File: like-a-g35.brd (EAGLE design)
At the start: 100 x 80 mm, 17 parts, among them J1 AVR_SPI_PRG_62X3_LOCK, Q1 16MHz, X1 S1, X2 S2, X3 S3, X4 POWER

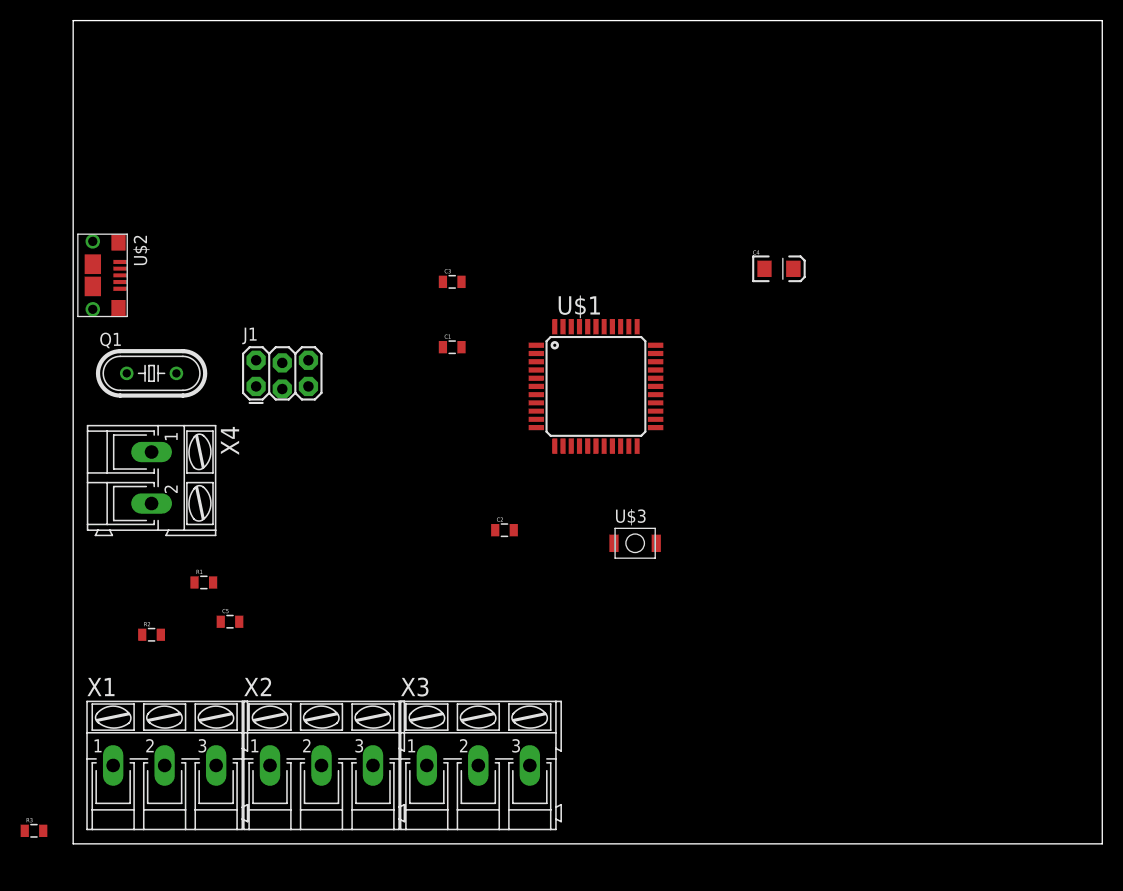
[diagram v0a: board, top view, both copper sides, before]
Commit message: 0.9.
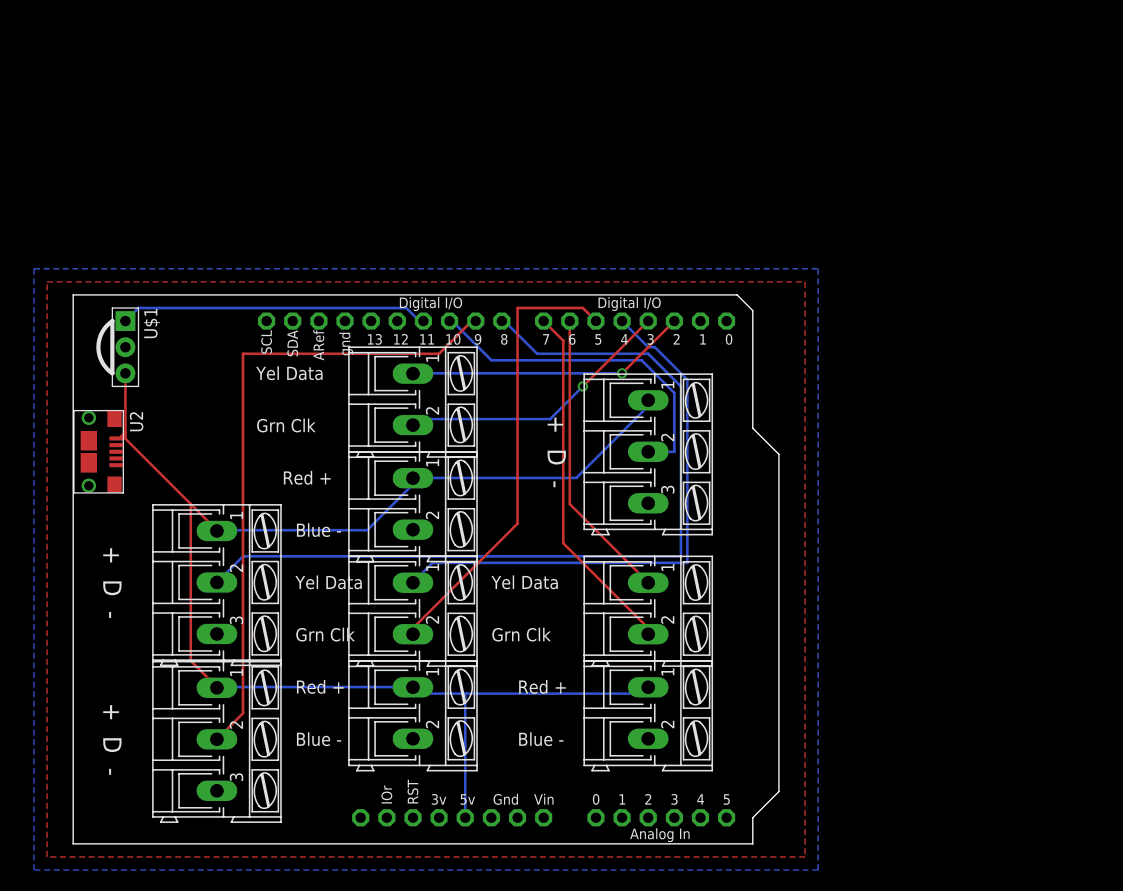
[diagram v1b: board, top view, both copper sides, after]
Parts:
- removed C1, C2: 18pF, programmer:0805
- removed C3, C5: 0.1uF, programmer:0805
- removed C4: 10uF, programmer:EIA3216
- removed J1: AVR_SPI_PRG_62X3_LOCK, programmer:2X3_LOCK
- removed Q1: 16MHz, crystal:HC49/S
- removed R1, R2: 22, like-a-g35:0805
- removed R3: 10K, like-a-g35:0805
- removed U$2: FCI_8193_MICRO_USB, programmer:FCI_MICRO_USB_8193
- removed U$3: BUTTON_TD-85XU, programmer:BUTTON_TD-85XU
- added U1: ARDUINOR3-DIMENSION, adafruit:ARDUINOR3
- added U2: FCI_8193_MICRO_USB, programmer:FCI_MICRO_USB_8193
- added X5, X6: POWER, con-ptr500:AK300/2
- added X7: WS1, con-ptr500:AK300/2
- added X8: WS2, con-ptr500:AK300/2
- added X9: WS3, con-ptr500:AK300/2
- U$1: value ATMEGA32U4-AU -> PNA460XM; device like-a-g35:TQFP44 -> adafruit:PNA460XM
- X1: value S1 -> G1
- X2: value S2 -> G2
- X3: value S3 -> G3
- moved U$1 45.9 mm to (5.08, 48.3), turned to 270 degrees
- moved X3 34.7 mm to (55.9, 38.1), turned to 270 degrees
- moved X4 25.5 mm to (33.0, 33.0)
- moved X1 18.5 mm to (14.0, 25.4), turned to 270 degrees
- moved X2 10.5 mm to (14.0, 10.2), turned to 270 degrees
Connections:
- removed net !RESET: J1.5, U$1.13
- removed net 3V3: C5.1, U$1.6
- removed net D+: R2.2, U$1.4
- removed net D-: R1.2, U$1.3
- removed net MISO: J1.1, U$1.11
- removed net MOSI: J1.4, U$1.10
- removed net N$1: R3.1, U$1.33, U$3.PAD1
- removed net RAW_D+: R2.1, U$2.D+
- removed net RAW_D-: R1.1, U$2.D-
- removed net SCK: J1.3, U$1.9
- removed net XTAL1: C1.1, Q1.2, U$1.17
- removed net XTAL2: C2.1, Q1.1, U$1.16
- new net 3V: U1.3V
- new net CLK1: U1.D3, X7.2
- new net CLK2: U1.D5, X8.2
- new net CLK3: U1.D7, X9.2
- new net DATA1: U1.D2, X7.1
- new net DATA2: U1.D4, X8.1
- new net DATA3: U1.D6, X9.1
- new net GDATA1: U1.D8, X1.2
- new net GDATA2: U1.D9, X2.2
- new net GDATA3: U1.D10, X3.2
- new net IR-OUT: U$1.1, U1.D11
- new net VIN: U1.VIN
- net +5V: now also U$1.3, U1.5V, U2.VBUS, X5.1, X6.1; no longer C3.1, C4.A, J1.2, R3.2, U$1.14, U$1.2, U$1.24, U$1.34, U$1.44, U$1.7, U$2.VBUS
- net GND: now also U$1.2, U1.GND, U1.GND1, U1.GND2, U2.GND, X5.2, X6.2; no longer C1.2, C2.2, C3.2, C4.C, C5.2, J1.6, U$1.15, U$1.23, U$1.35, U$1.43, U$1.5, U$2.GND, U$3.PAD2
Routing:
- net +5V: track 0.00 -> 142.3 mm
- net GDATA1: track 0.00 -> 82.7 mm
- net GDATA2: track 0.00 -> 62.4 mm
- net DATA2: track 0.00 -> 54.0 mm
- net CLK2: track 0.00 -> 44.1 mm
- net CLK3: track 0.00 -> 34.6 mm
- net GDATA3: track 0.00 -> 33.0 mm
- net IR-OUT: track 0.00 -> 30.0 mm
- net DATA3: track 0.00 -> 28.6 mm
- net DATA1: track 0.00 -> 27.5 mm, vias 0 -> 1
- net CLK1: track 0.00 -> 27.4 mm, vias 0 -> 1
- added copper zone on layer 1, net GND
- added copper zone on layer 16, net GND
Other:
- board size 100 x 80 mm -> 68.6 x 53.3 mm
- board text added: "+ D -"
- board text added: "Blue -"
- board text added: "Grn Clk"
- board text added: "Red +"
- board text added: "Yel Data"
